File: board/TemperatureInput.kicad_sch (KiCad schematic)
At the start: 18 parts, among them U4 OPA2134, U8 TL431DBZ, U9 OPA2134

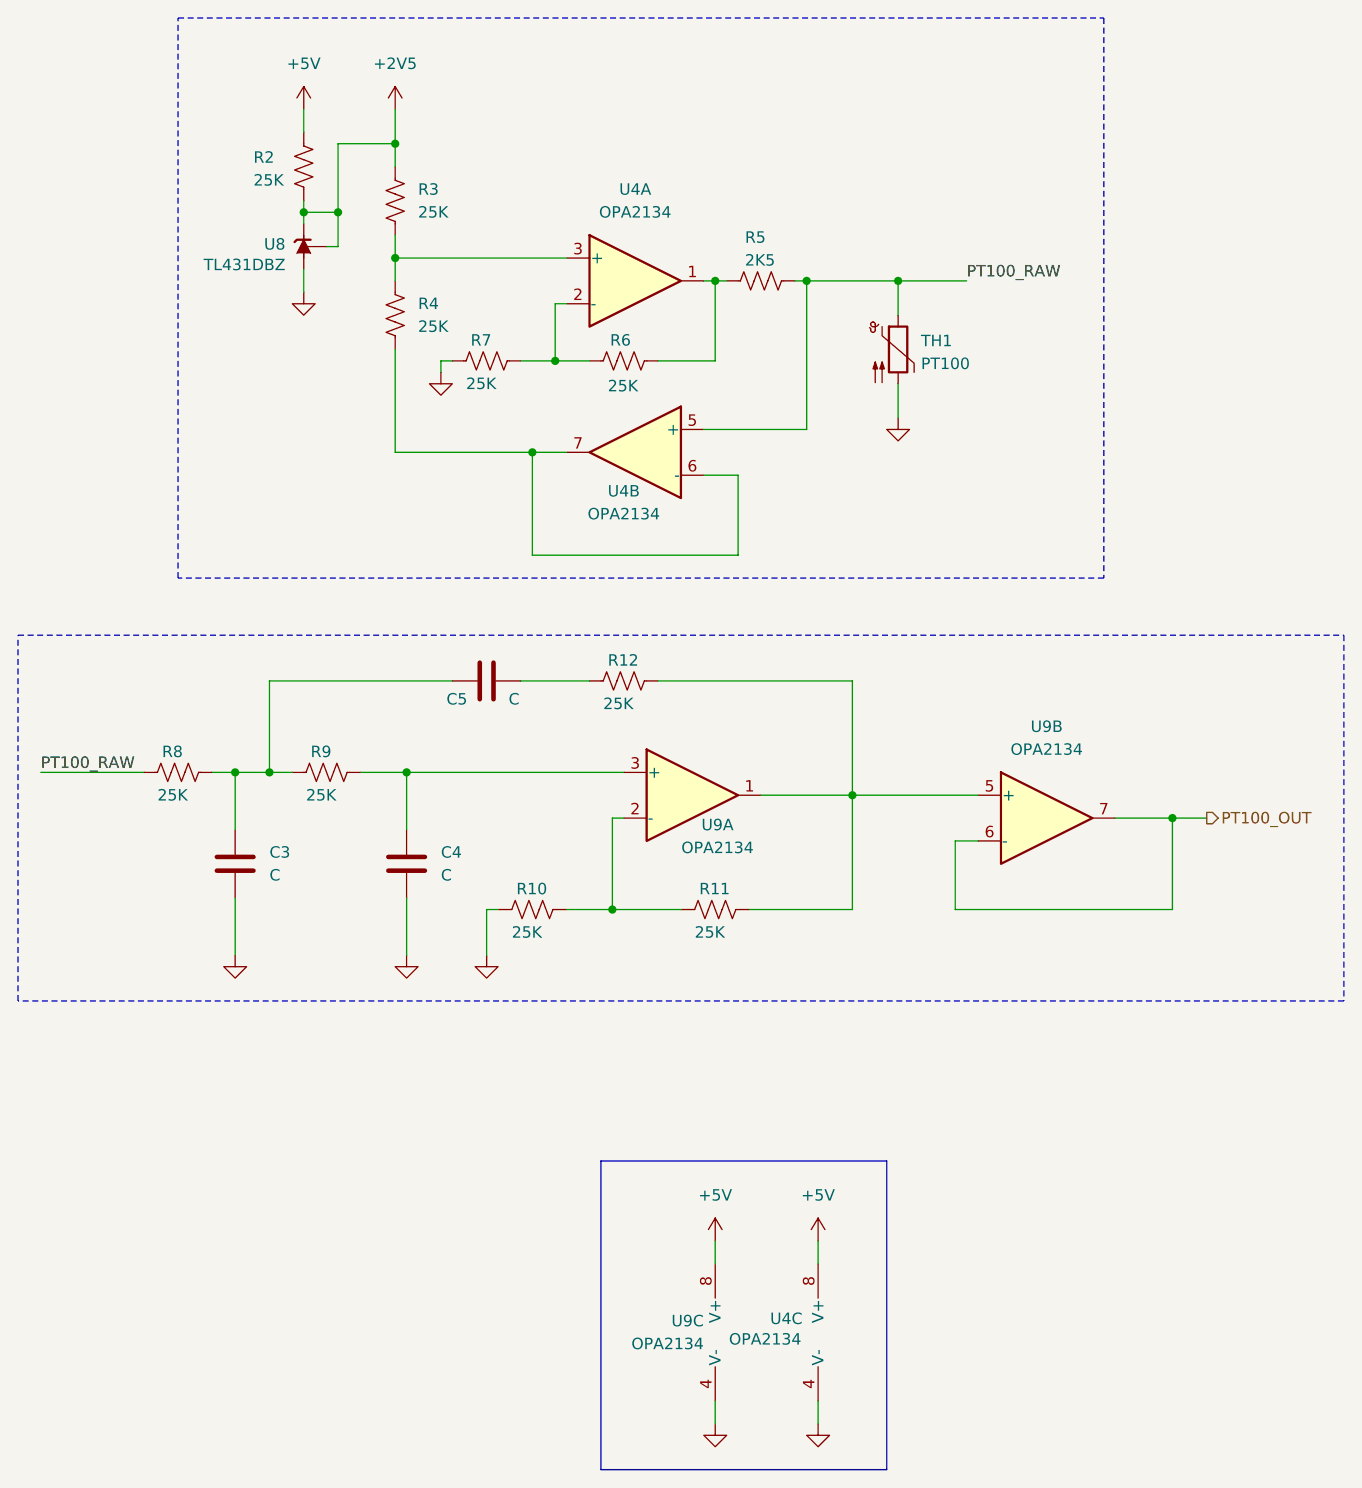
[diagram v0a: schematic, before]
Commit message: [6-5-2024] Create I/O
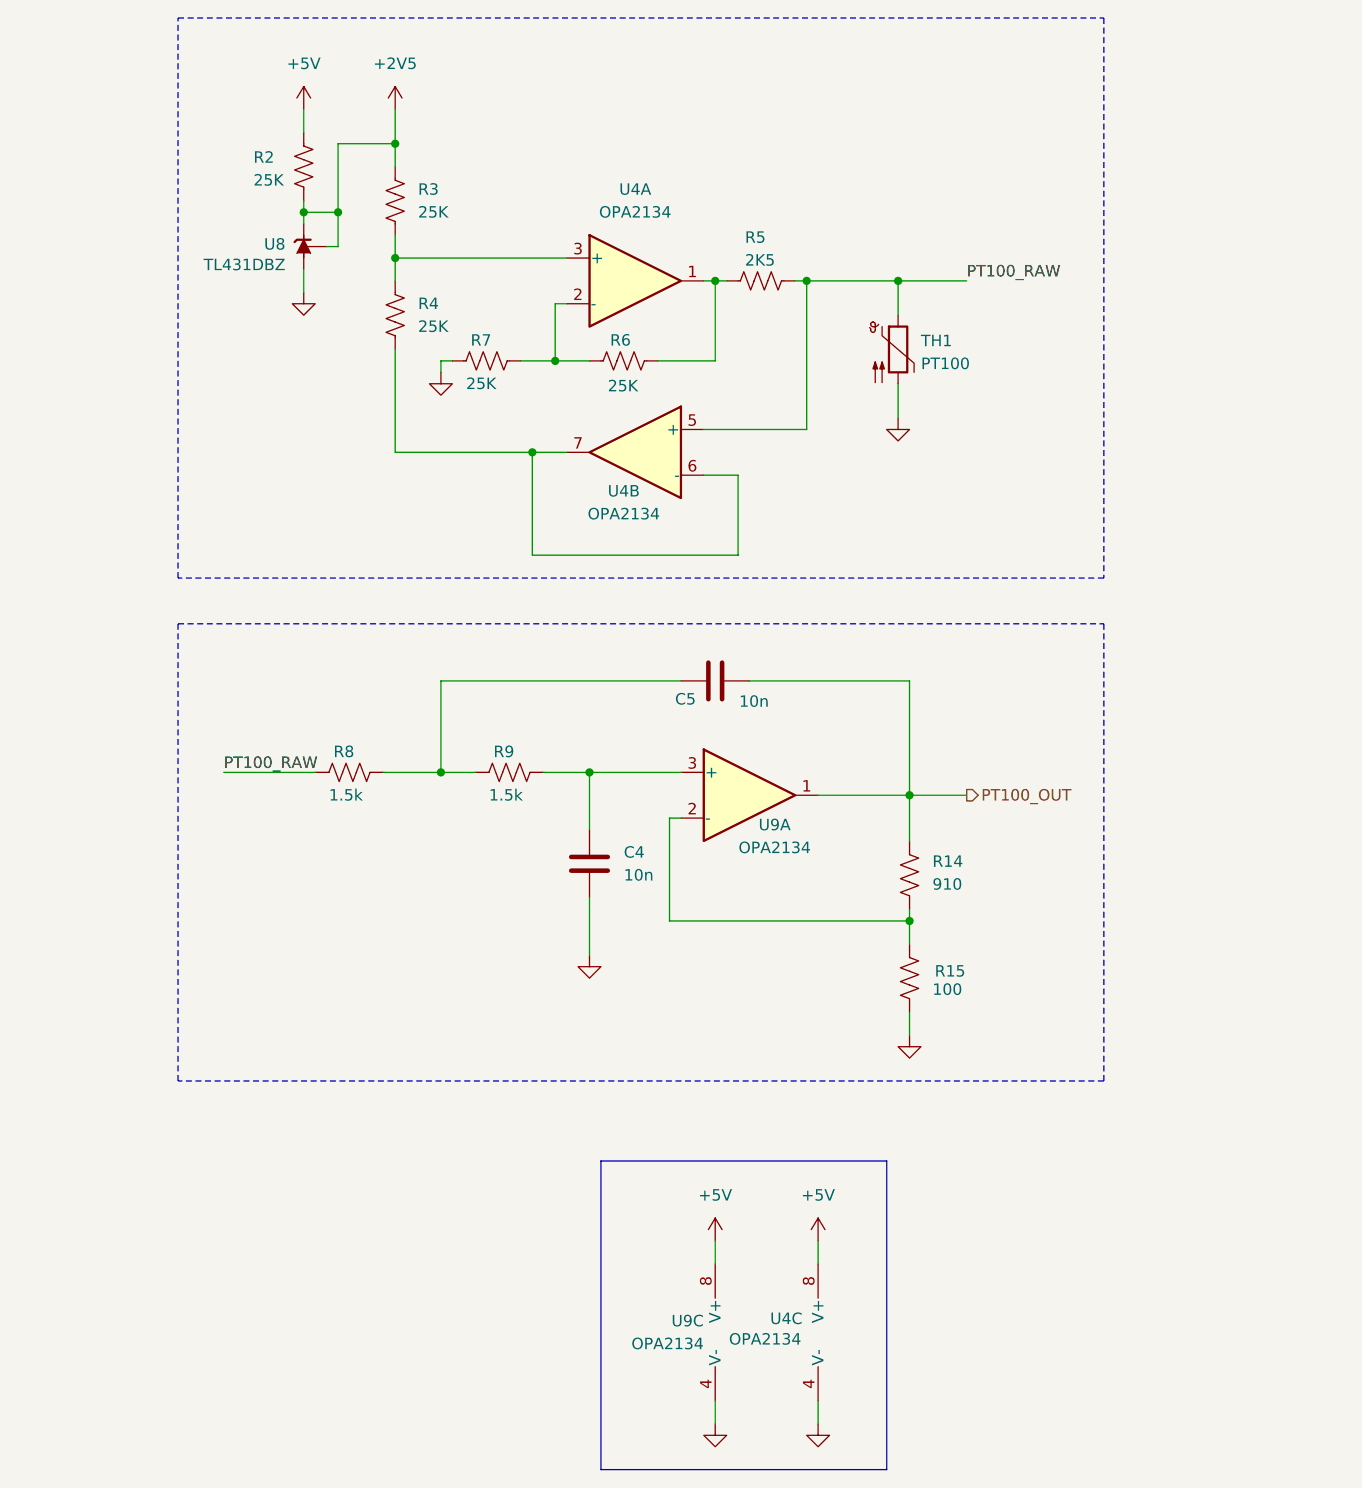
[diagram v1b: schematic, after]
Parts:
- removed C3: C, Capacitor_SMD:C_01005_0402Metric_Pad0.57x0.30mm_HandSolder, symbol Device:C
- removed R10, R11, R12: 25K, Resistor_SMD:R_0805_2012Metric_Pad1.20x1.40mm_HandSolder, symbol Device:R_US
- removed unit 2 of U9
- added R14: 910, Resistor_SMD:R_0805_2012Metric_Pad1.20x1.40mm_HandSolder, symbol Device:R_US
- added R15: 100, Resistor_SMD:R_0805_2012Metric_Pad1.20x1.40mm_HandSolder, symbol Device:R_US
- C4, C5: value C -> 10n
- R8, R9: value 25K -> 1.5k
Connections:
- net GND: now also R15.2
- net PT100_OUT: now also C5.2, U9.1, R14.1
- net at U9.2 (-): now also R14.2, R15.1
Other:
- moved on the sheet: C4, C5, R8, R9, U9A
